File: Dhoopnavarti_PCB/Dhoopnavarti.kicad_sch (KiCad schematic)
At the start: 12 parts, among them J1 Conn_01x04_Pin, J2 Conn_01x05_Pin, J3 Conn_01x04_Pin, J5 USB_A, SW1 Screw_Terminal_01x02, U1 NUCLEO-L432KC, U2 LM7805_TO220

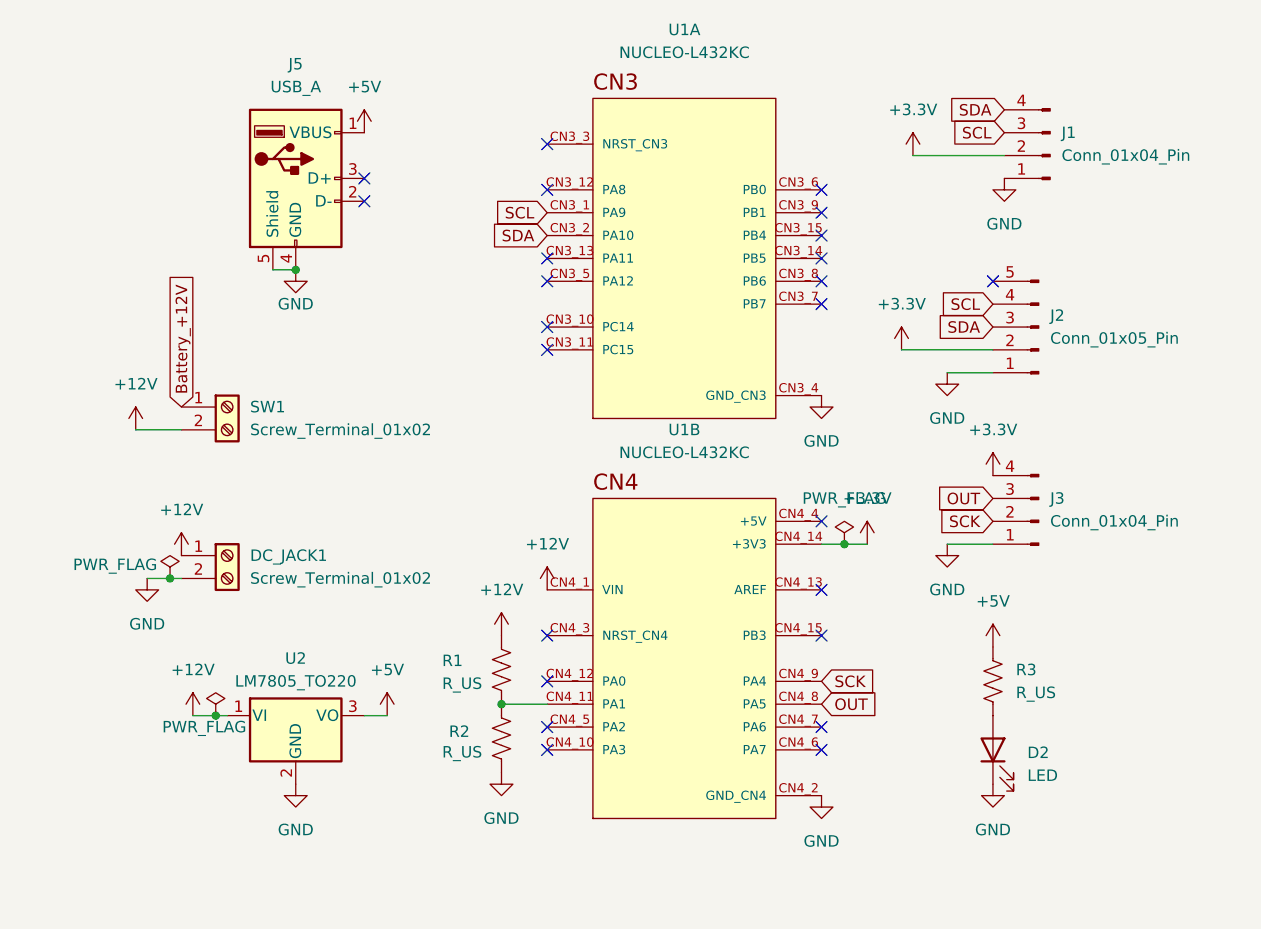
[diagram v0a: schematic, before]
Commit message: Routing v1
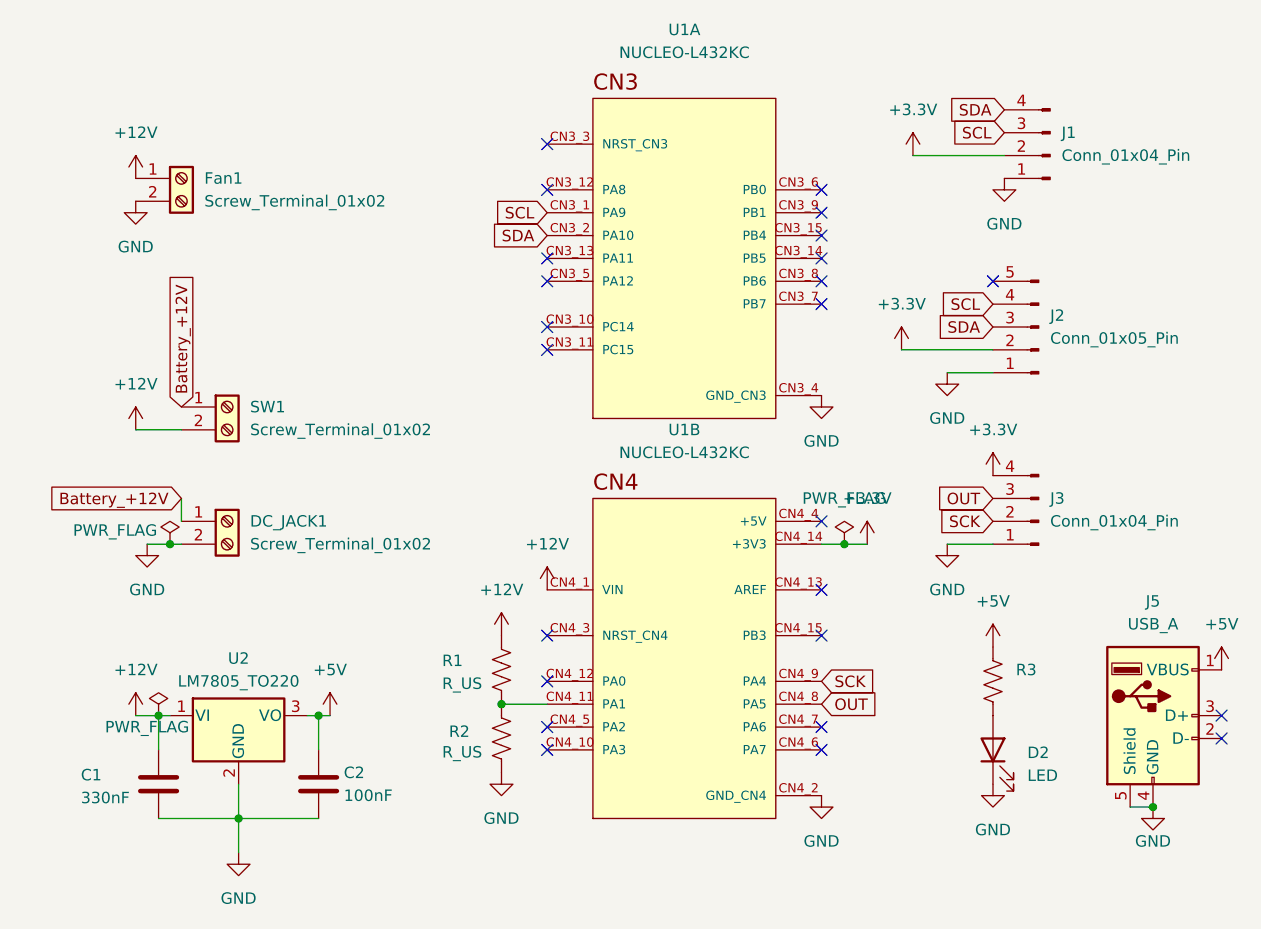
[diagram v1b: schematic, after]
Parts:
- added C1: 330nF, Capacitor_THT:C_Disc_D3.4mm_W2.1mm_P2.50mm, symbol Device:C
- added C2: 100nF, Capacitor_THT:C_Disc_D3.4mm_W2.1mm_P2.50mm, symbol Device:C
- added Fan1: Screw_Terminal_01x02, Custom_Footprints:Wire_Pad, symbol Connector:Screw_Terminal_01x02
- D2: footprint (none) -> LED_THT:LED_D3.0mm
- J1, J3: footprint Connector_PinHeader_2.54mm:PinHeader_1x04_P2.54mm_Vertical -> Connector_JST:JST_XH_B4B-XH-A_1x04_P2.50mm_Vertical
- J2: footprint Connector_PinHeader_2.54mm:PinHeader_1x05_P2.54mm_Vertical -> Connector_JST:JST_XH_B5B-XH-A_1x05_P2.50mm_Vertical
- R1, R2: footprint (none) -> Resistor_THT:R_Axial_DIN0207_L6.3mm_D2.5mm_P10.16mm_Horizontal
- R3: value R_US -> 220; footprint (none) -> Resistor_THT:R_Axial_DIN0207_L6.3mm_D2.5mm_P10.16mm_Horizontal
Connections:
- net +12V: now also C1.1, Fan1.1 (Pin_1); no longer DC_JACK1.1 (Pin_1)
- net +5V: now also C2.1
- net Battery_+12V: now also DC_JACK1.1 (Pin_1)
- net GND: now also C1.2, C2.2, Fan1.2 (Pin_2)
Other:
- moved on the sheet: DC_JACK1, J5, U2
